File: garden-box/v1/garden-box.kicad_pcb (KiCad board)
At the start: 2 copper layers, 88.9 x 66 mm, 0 parts

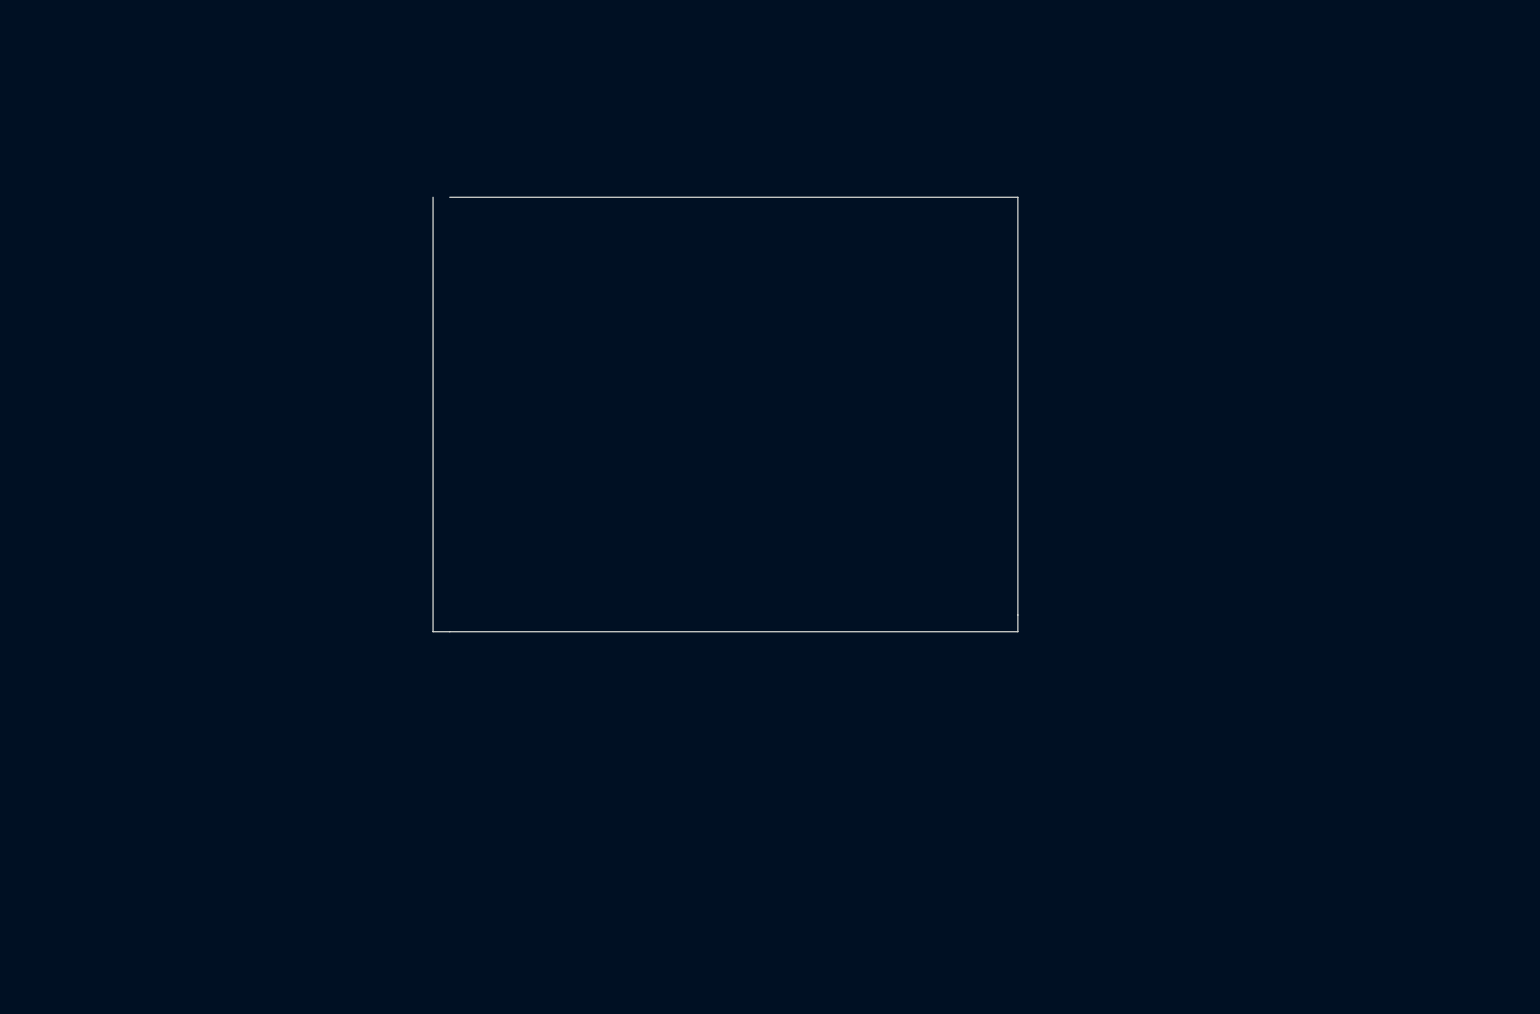
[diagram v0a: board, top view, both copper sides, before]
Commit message: init new v1
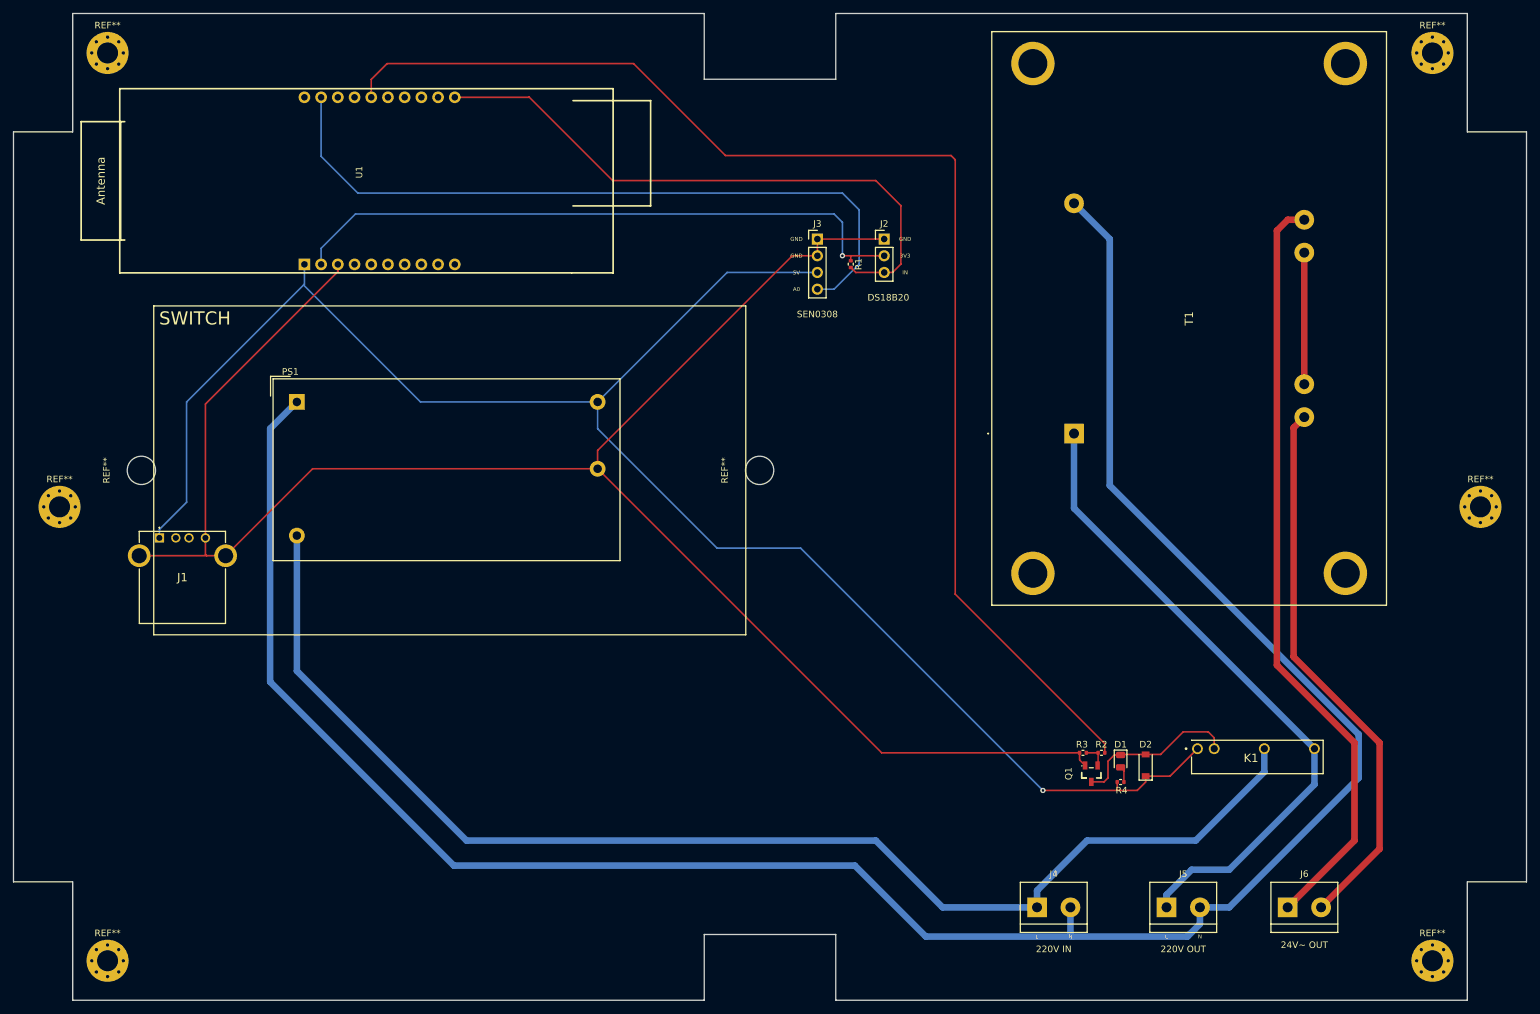
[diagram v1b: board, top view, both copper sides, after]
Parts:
- added D1: LED, Diode_SMD:D_0805_2012Metric, F.Cu at (198.5, 128.9)
- added D2: 1N4148, Diode_SMD:D_SOD-123, F.Cu at (202.3, 129.5)
- added J1: USB_A, rs-online:875200010BLF, F.Cu at (52.4, 95.0)
- added J2: Conn_01x03_Male, Connector_PinHeader_2.54mm:PinHeader_1x03_P2.54mm_Vertical, F.Cu at (162.6, 49.5)
- added J3: Conn_01x04_Male, Connector_PinHeader_2.54mm:PinHeader_1x04_P2.54mm_Vertical, F.Cu at (152.4, 49.5)
- added J4: Screw_Terminal_01x02, TerminalBlock:TerminalBlock_bornier-2_P5.08mm, F.Cu at (185.8, 151.1)
- added J5: Screw_Terminal_01x02, TerminalBlock:TerminalBlock_bornier-2_P5.08mm, F.Cu at (205.5, 151.1)
- added J6: Screw_Terminal_01x02, TerminalBlock:TerminalBlock_bornier-2_P5.08mm, F.Cu at (223.9, 151.1)
- added K1: G6DN-1A-L_DC5, rs-online:G6DN-1A-L, F.Cu at (228.0, 127.0)
- added PS1: RS PRO 5V 2A, mylife-footprints:RS PRO 5V 2A, F.Cu at (73.3, 74.3)
- added Q1: 2N3904, jlcpcb:SOT-23-3_L2.9-W1.3-P1.90-LS2.4-TR, F.Cu at (194.0, 130.8)
- added R1: 4.7KΩ, Resistor_SMD:R_0402_1005Metric, F.Cu at (157.5, 53.3)
- added R2: 1KΩ, Resistor_SMD:R_0402_1005Metric, F.Cu at (195.6, 127.6)
- added R3: 10KΩ, Resistor_SMD:R_0402_1005Metric, F.Cu at (192.8, 127.6)
- added R4: 330Ω, Resistor_SMD:R_0402_1005Metric, F.Cu at (198.5, 132.1)
- added REF**: MountingHole_3.2mm_M3_Pad_Via, MountingHole:MountingHole_3.2mm_M3_Pad_Via, F.Cu at (245.9, 159.2)
- added REF**: MountingHole_3.2mm_M3_Pad_Via, MountingHole:MountingHole_3.2mm_M3_Pad_Via, F.Cu at (44.5, 159.2)
- added REF**: MountingHole_3.2mm_M3_Pad_Via, MountingHole:MountingHole_3.2mm_M3_Pad_Via, F.Cu at (44.5, 21.2)
- added REF**: MountingHole_3.2mm_M3_Pad_Via, MountingHole:MountingHole_3.2mm_M3_Pad_Via, F.Cu at (37.2, 90.2)
- added REF**: MountingHole_3.2mm_M3_Pad_Via, MountingHole:MountingHole_3.2mm_M3_Pad_Via, F.Cu at (253.2, 90.2)
- added REF**: MountingHole_4.3mm_M4, MountingHole:MountingHole_4.3mm_M4, F.Cu at (143.6, 84.7)
- added REF**: MountingHole_4.3mm_M4, MountingHole:MountingHole_4.3mm_M4, F.Cu at (49.6, 84.7)
- added REF**: MountingHole_3.2mm_M3_Pad_Via, MountingHole:MountingHole_3.2mm_M3_Pad_Via, F.Cu at (245.9, 21.2)
- added T1: Transformer_1P_2S, rs-online:VCM36212, F.Cu at (191.4, 79.1)
- added U1: ESP32-POE, mylife-footprints:ESP32-POE, F.Cu at (84.5, 40.6)
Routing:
- net Net-(J4-Pad2): track 0.00 -> 347.0 mm
- net GND: track 0.00 -> 282.4 mm
- net +5V: track 0.00 -> 266.7 mm, vias 0 -> 1
- net Net-(R2-Pad2): track 0.00 -> 198.1 mm
- net Net-(J4-Pad1): track 0.00 -> 196.1 mm
- net Net-(J6-Pad1): track 0.00 -> 116.8 mm
- net Net-(J3-Pad4): track 0.00 -> 110.3 mm
- net Net-(J5-Pad1): track 0.00 -> 99.8 mm
- net +3V3: track 0.00 -> 96.6 mm, vias 0 -> 1
- net Net-(J2-Pad3): track 0.00 -> 92.0 mm
- net Net-(J6-Pad2): track 0.00 -> 84.3 mm
- net Net-(D1-Pad1): track 0.00 -> 25.3 mm
- net Net-(T1-Pad4): track 0.00 -> 20.0 mm
- net Net-(Q1-Pad2): track 0.00 -> 3.74 mm
- net Net-(D1-Pad2): track 0.00 -> 2.45 mm
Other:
- board size 88.9 x 66 mm -> 230 x 150 mm
- board text added: "220V IN"
- board text added: "220V OUT"
- board text added: "24V~ OUT"
- board text added: "3V3"
- board text added: "5V"
- board text added: "A0"
- board text added: "DS18B20"
- board text added: "GND"
- board text added: "IN"
- board text added: "L"
- board text added: "N"
- board text added: "SEN0308"
- board text added: "SWITCH"
